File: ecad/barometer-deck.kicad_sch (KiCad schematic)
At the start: 28 parts, among them IC1 MIC5353-3.3YMT-TR, IC2 BMP390, P1 CF_EXP_LEFT, P2 CF_EXP_RIGHT, U1 NINA-W106-10B, U2 DS2431

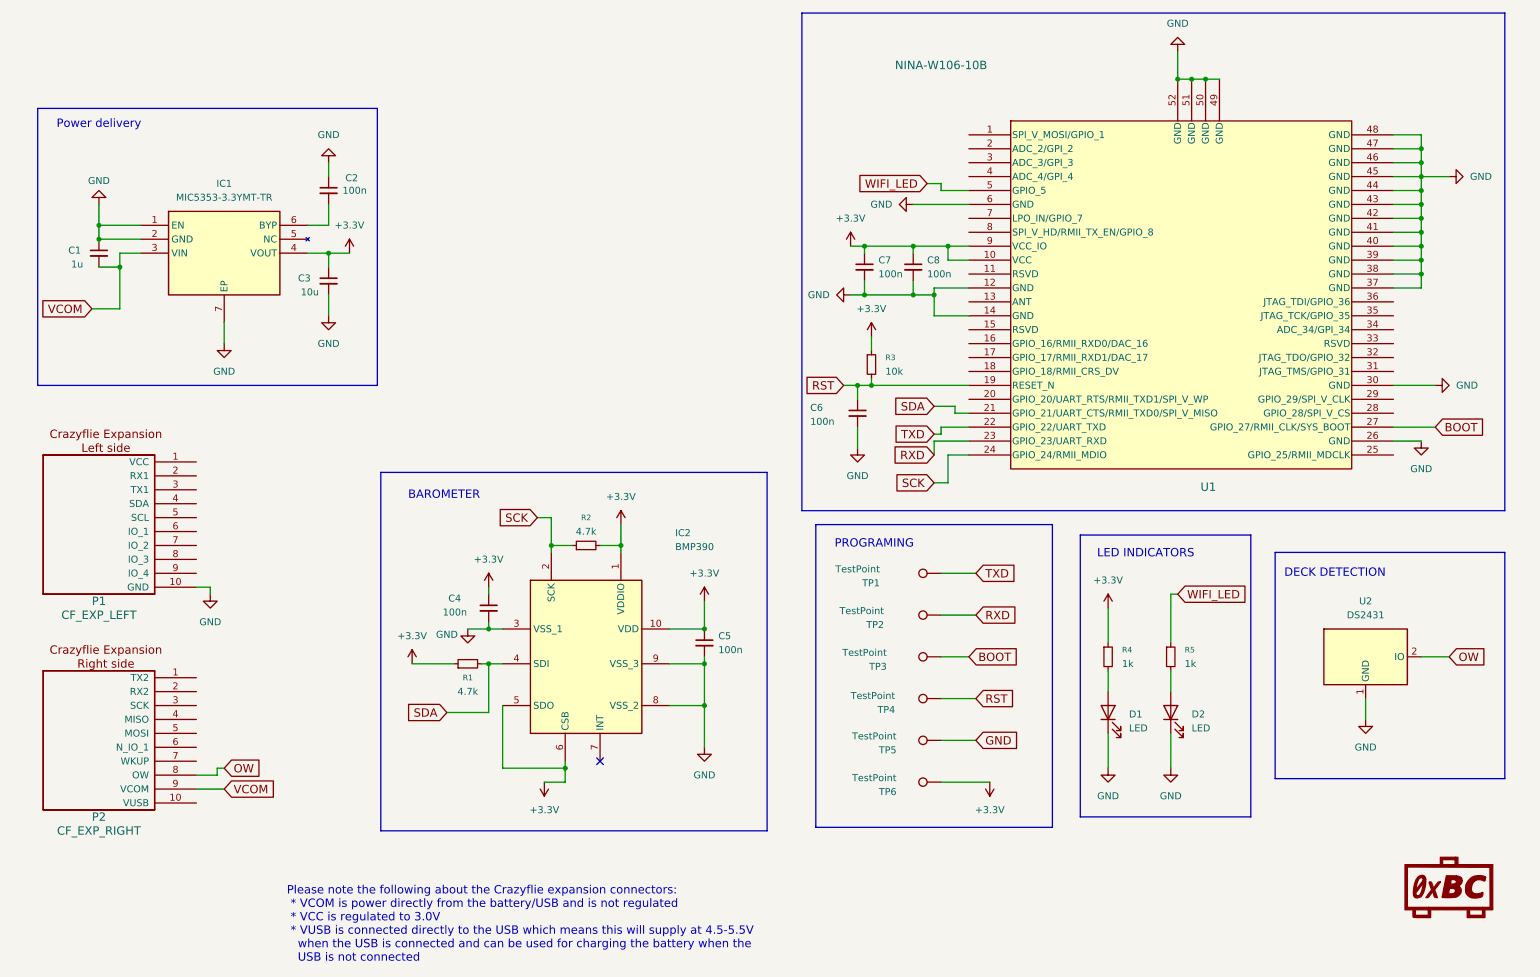
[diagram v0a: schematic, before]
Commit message: jtag support
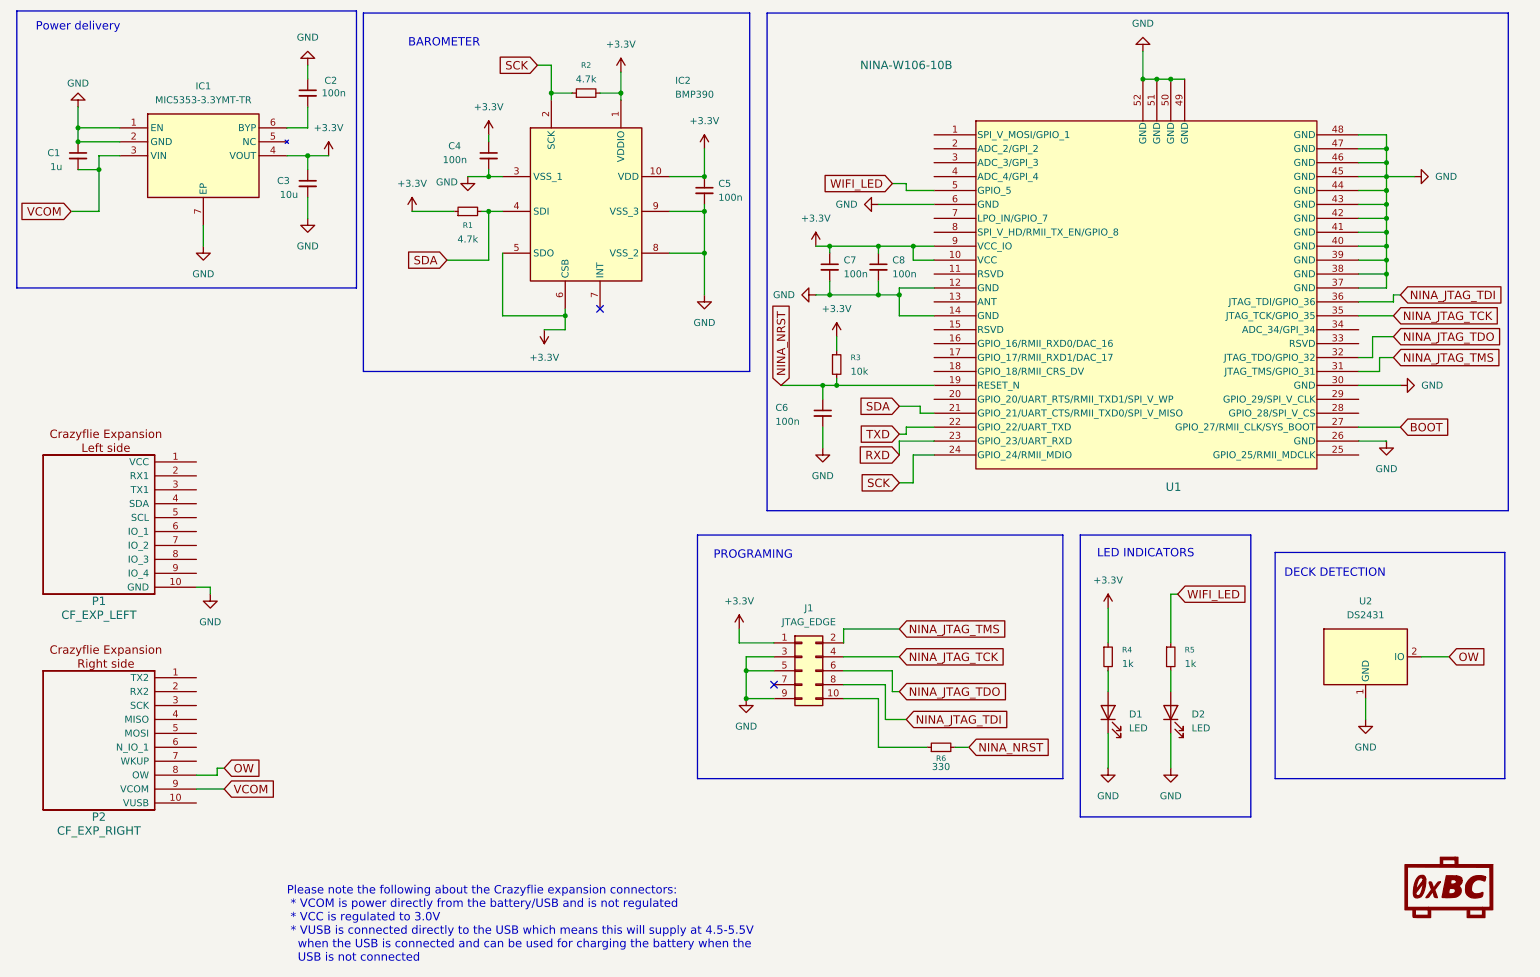
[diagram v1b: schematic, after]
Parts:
- removed TP1, TP2, TP3, TP4, TP5, TP6: TestPoint, Connector_PinHeader_2.54mm:PinHeader_1x01_P2.54mm_Vertical, symbol Connector:TestPoint
- added J1: JTAG_EDGE, Connector_PinHeader_1.27mm:PinHeader_2x05_P1.27mm_Horizontal, symbol Connector_Generic:Conn_02x05_Odd_Even
- added R6: 330, symbol Device:R_Small
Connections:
- net +3.3V: now also J1.1 (Pin_1)
- net GND: now also J1.3 (Pin_3), J1.5 (Pin_5), J1.9 (Pin_9)
- net NINA_JTAG_TMS: now reaches U1.31 (JTAG_TMS/GPIO_31)
- net NINA_JTAG_TMS: now also J1.2 (Pin_2)
- net NINA_JTAG_TDO: now reaches U1.32 (JTAG_TDO/GPIO_32)
- net NINA_JTAG_TDO: now also J1.6 (Pin_6)
- net NINA_JTAG_TCK: now reaches U1.35 (JTAG_TCK/GPIO_35)
- net NINA_JTAG_TCK: now also J1.4 (Pin_4)
- net NINA_JTAG_TDI: now reaches U1.36 (JTAG_TDI/GPIO_36)
- net NINA_JTAG_TDI: now also J1.8 (Pin_8)
- net RST renamed NINA_NRST
- net NINA_NRST: now also R6.2
- new net: J1.10 (Pin_10), R6.1
- no-connect marks 1 -> 2
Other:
- moved on the sheet: C1, C2, C3, C4, C5, C6, C7, C8, IC1, IC2, R1, R2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
